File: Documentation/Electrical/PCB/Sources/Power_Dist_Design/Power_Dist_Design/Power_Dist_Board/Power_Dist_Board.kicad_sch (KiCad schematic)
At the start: 47 parts, among them J1 Battery Connector, J2 5V Connector, J3 3.3V Connector, M1 Motor_DC, M2 Motor_DC, M3 Motor_DC, M4 Motor_DC, M5 Motor_DC, M6 Motor_DC, SW1 Emergency Stop, U1 TPS565201, U2 TPS565201

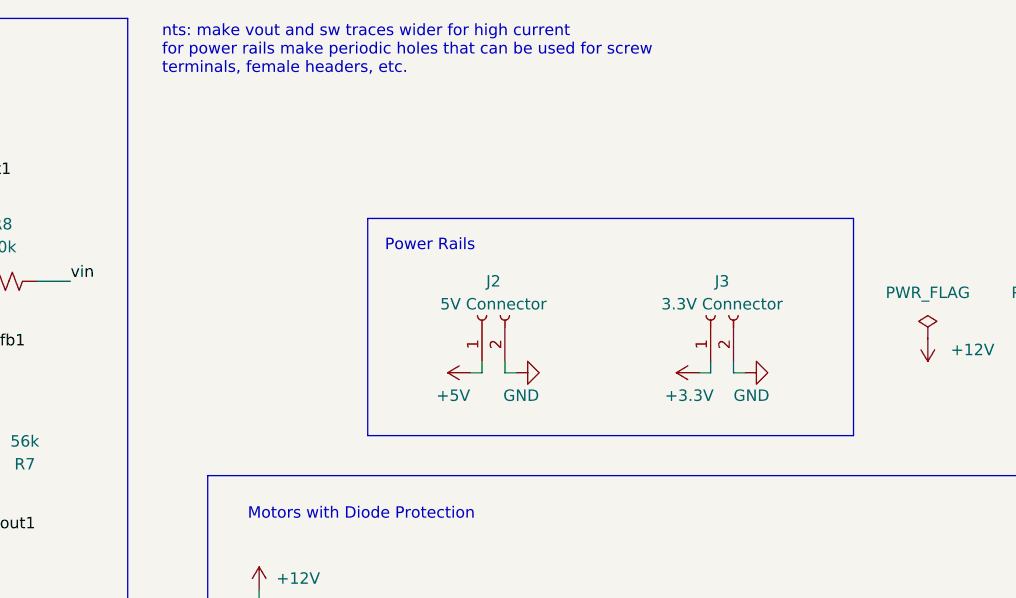
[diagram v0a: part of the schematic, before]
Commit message: Made further edits to pcb
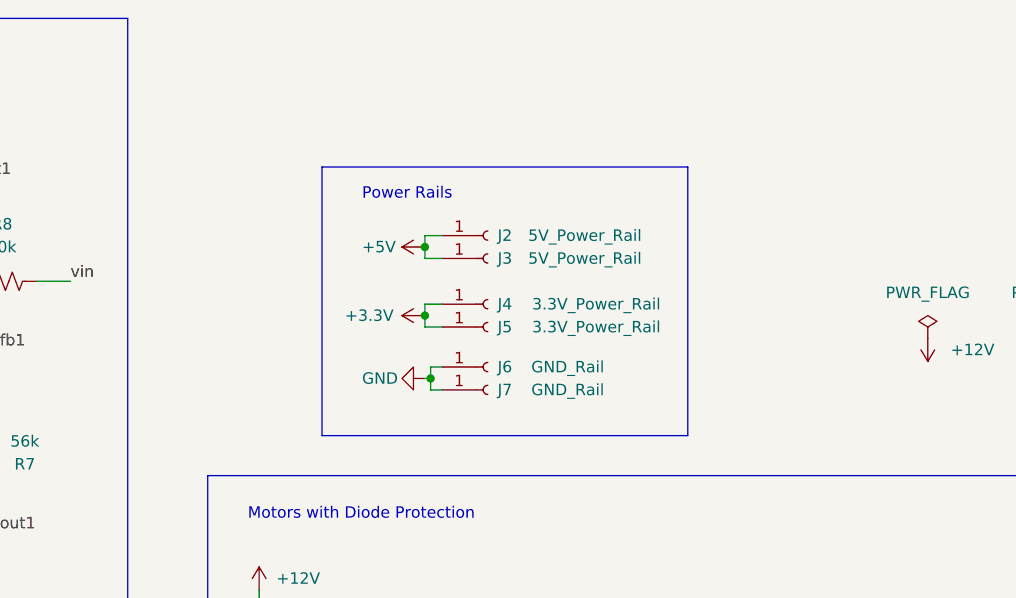
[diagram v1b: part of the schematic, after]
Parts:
- removed J2: 5V Connector, Connector_Phoenix_MSTB:PhoenixContact_MSTBVA_2,5_2-G-5,08_1x02_P5.08mm_Vertical, symbol Connector:Conn_01x02_Female
- removed J3: 3.3V Connector, Connector_Phoenix_MSTB:PhoenixContact_MSTBVA_2,5_2-G-5,08_1x02_P5.08mm_Vertical, symbol Connector:Conn_01x02_Female
- added J2, J3: 5V_Power_Rail, Power_Dist:Pwr_Rail_Conn_Custom, symbol Connector:Conn_01x01_Female
- added J4, J5: 3.3V_Power_Rail, Power_Dist:Pwr_Rail_Conn_Custom, symbol Connector:Conn_01x01_Female
- added J6, J7: GND_Rail, Power_Dist:Pwr_Rail_Conn_Custom, symbol Connector:Conn_01x01_Female
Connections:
- net +3.3V: now also J4.1 (Pin_1), J5.1 (Pin_1)
- net +5V: now also J2.1 (Pin_1), J3.1 (Pin_1)
- net GND: now also J6.1 (Pin_1), J7.1 (Pin_1)
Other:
- note removed: "nts: make vout and sw traces wider for high current for power rails make periodic holes that can be used for screw terminals, female headers, etc."
